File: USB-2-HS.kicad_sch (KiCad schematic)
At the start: 18 parts, among them J900 U-M-M5DW-W-1, U900 USB3320C-EZK-TR, X900 ECS-2520MV-130-BN

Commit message: ram-update
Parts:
- FB900: footprint FB_0402 -> Footprint-Lib-PhilsLab:FB_0402
- U900: footprint QFN-32-5x5x0.85mm -> Footprint-Lib-PhilsLab:QFN-32-5x5x0.85mm
- X900: footprint XTAL_2520 -> Footprint-Lib-PhilsLab:XTAL_2520
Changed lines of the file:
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@@
 			)
 		)
-		(property "Footprint" "QFN-32-5x5x0.85mm"
+		(property "Footprint" "Footprint-Lib-PhilsLab:QFN-32-5x5x0.85mm"
 			(at 128.27 86.36 0)
 			(effects
@@
 			)
 		)
-		(property "Footprint" "FB_0402"
+		(property "Footprint" "Footprint-Lib-PhilsLab:FB_0402"
 			(at 212.09 63.5 0)
 			(effects
@@
 			)
 		)
-		(property "Footprint" "XTAL_2520"
+		(property "Footprint" "Footprint-Lib-PhilsLab:XTAL_2520"
 			(at 43.18 104.14 0)
 			(effects

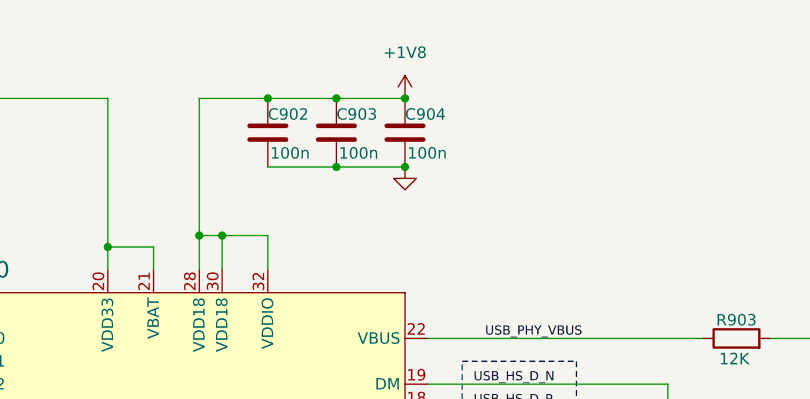
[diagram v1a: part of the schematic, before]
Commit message: ram-zynq-updated
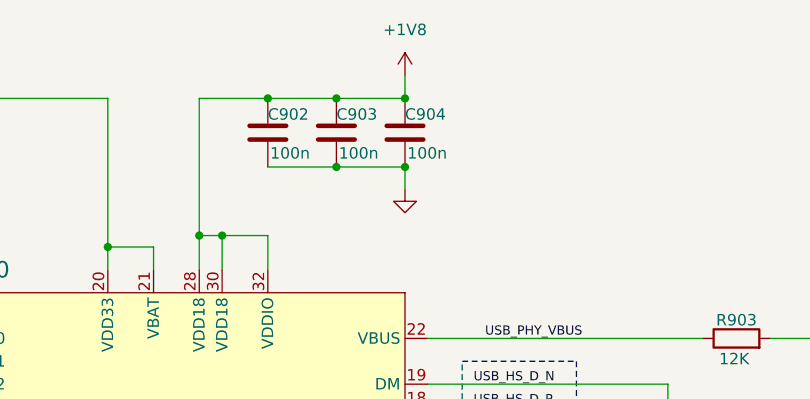
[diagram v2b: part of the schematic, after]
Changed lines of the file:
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@@
+	(wire
+		(pts
+			(xy 153.67 46.99) (xy 153.67 44.45)
+		)
+		(stroke
+			(width 0)
+			(type default)
+		)
+	)
 	(wire
 		(pts
@@
 		(pts
 			(xy 158.75 101.6) (xy 156.21 101.6)
+		)
+		(stroke
+			(width 0)
+			(type default)
+		)
+	)
+	(wire
+		(pts
+			(xy 153.67 34.29) (xy 153.67 36.83)
 		)
 		(stroke
@@
 	(symbol
 		(lib_id "power:+1V0")
-		(at 153.67 36.83 0)
+		(at 153.67 34.29 0)
 		(unit 1)
 		(exclude_from_sim no)
@@
 		(fields_autoplaced yes)
 		(property "Reference" "#PWR0198"
-			(at 153.67 40.64 0)
+			(at 153.67 38.1 0)
 			(effects
 				(font
@@
 		)
 		(property "Value" "+1V8"
-			(at 153.67 31.75 0)
+			(at 153.67 29.21 0)
 			(effects
 				(font
@@
 		)
 		(property "Footprint" ""
-			(at 153.67 36.83 0)
+			(at 153.67 34.29 0)
 			(effects
 				(font
@@
 		)
 		(property "Datasheet" ""
-			(at 153.67 36.83 0)
+			(at 153.67 34.29 0)
 			(effects
 				(font
@@
 		)
 		(property "Description" "Power symbol creates a global label with name \"+1V0\""
-			(at 153.67 36.83 0)
+			(at 153.67 34.29 0)
 			(effects
 				(font
@@
 	(symbol
 		(lib_id "power:GND")
-		(at 153.67 44.45 0)
+		(at 153.67 46.99 0)
 		(unit 1)
 		(exclude_from_sim no)
@@
 		(dnp no)
 		(property "Reference" "#PWR0195"
-			(at 153.67 50.8 0)
+			(at 153.67 53.34 0)
 			(effects
 				(font
@@
 		)
 		(property "Value" "GND"
-			(at 151.638 47.752 0)
+			(at 151.638 50.292 0)
 			(effects
 				(font
@@
 		)
 		(property "Footprint" ""
-			(at 153.67 44.45 0)
+			(at 153.67 46.99 0)
 			(effects
 				(font
@@
 		)
 		(property "Datasheet" ""
-			(at 153.67 44.45 0)
+			(at 153.67 46.99 0)
 			(effects
 				(font
@@
 		)
 		(property "Description" "Power symbol creates a global label with name \"GND\" , ground"
-			(at 153.67 44.45 0)
-			(effects
-				(font
+			(at 153.67 46.99 0)
+			(effects
+				(font
